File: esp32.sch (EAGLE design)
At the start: 28 parts, among them IC1 LM1117IMPX-3.3, U1 ESP32MOD

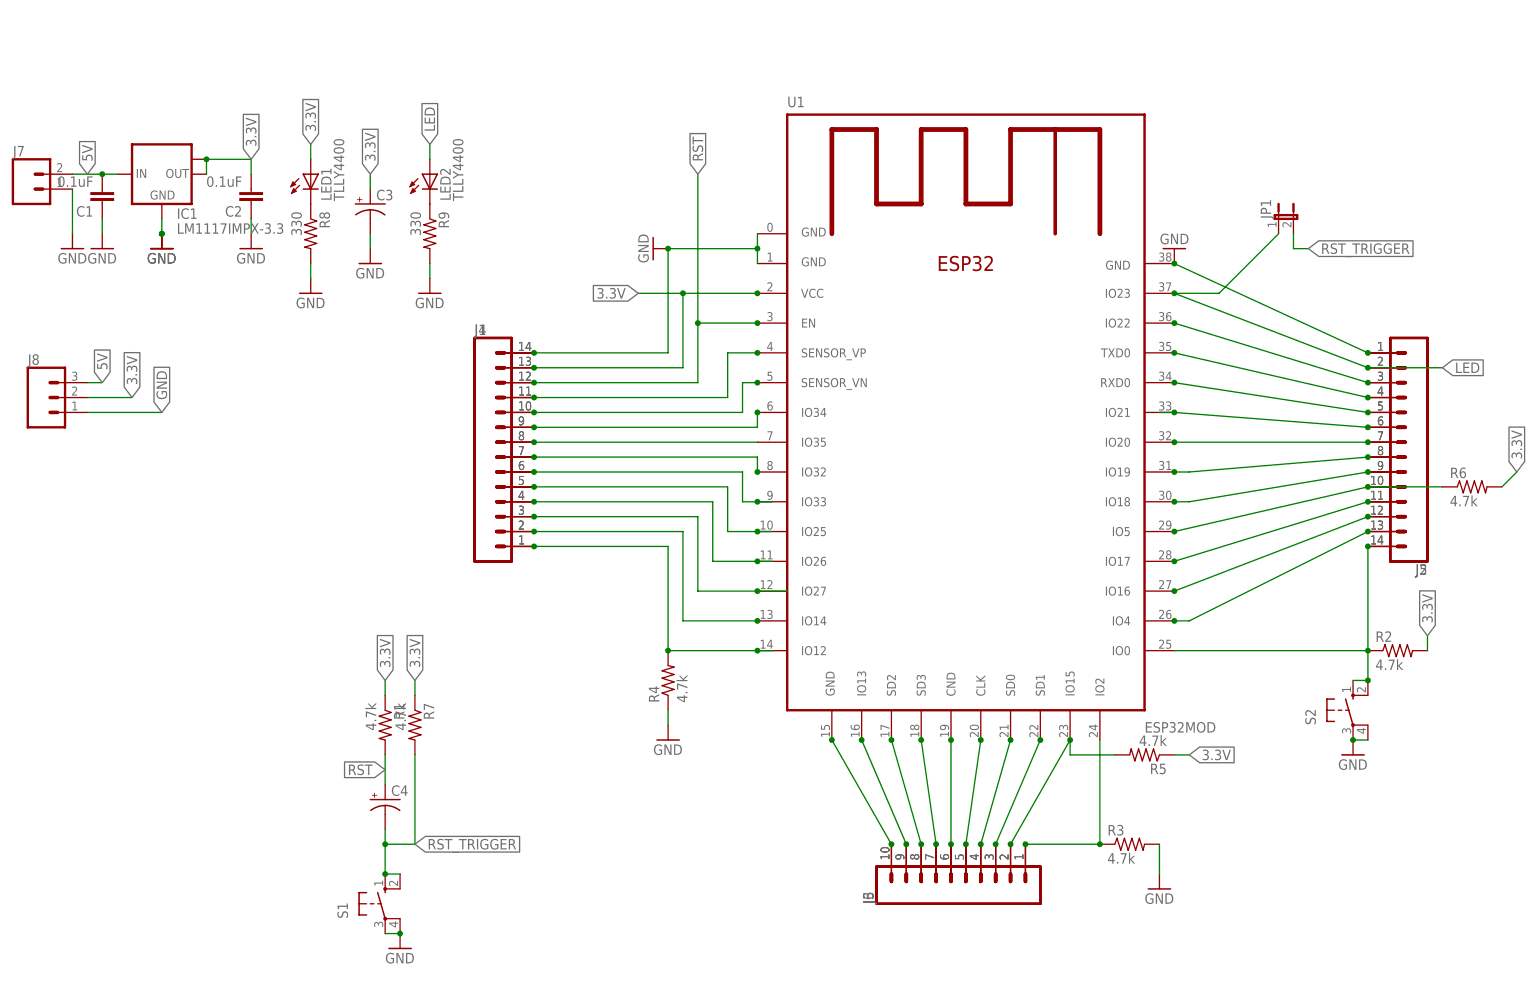
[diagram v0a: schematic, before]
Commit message: Finalized the layout with cheap design
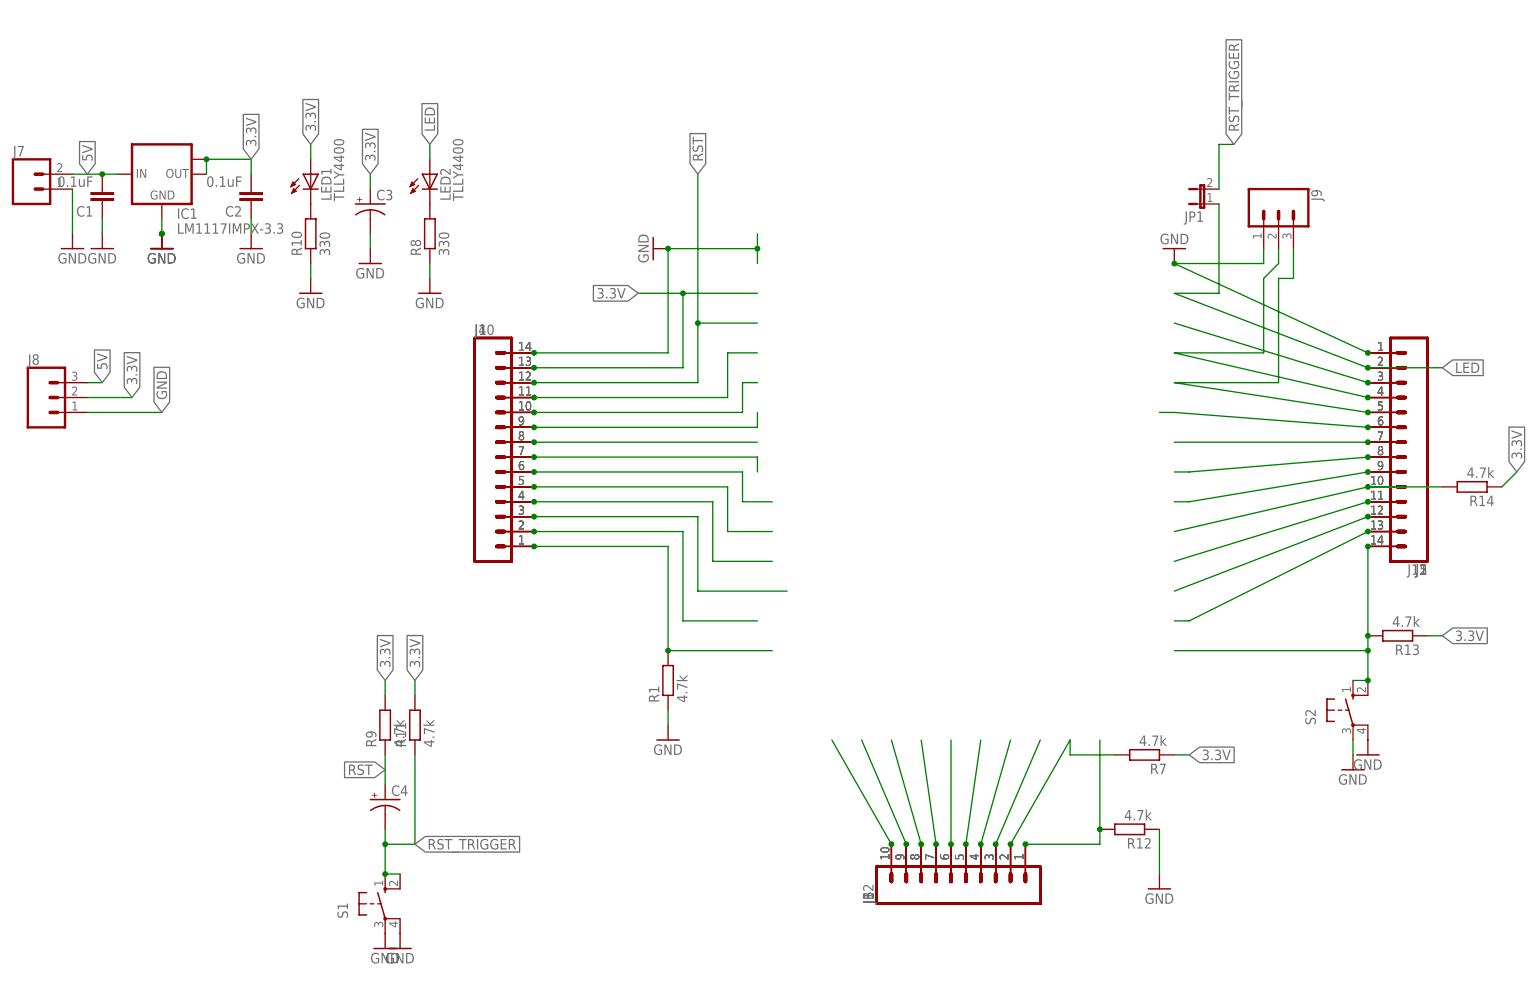
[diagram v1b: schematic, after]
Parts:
- removed R2, R3, R4, R5, R6: 4.7k, rcl:R-US_0411/15
- removed U1: ESP32MOD, ESP3x:ESP32MOD
- added J10, J11: (no value), SparkFun-Connectors:CONN_14LONGPADS
- added J12: (no value), SparkFun-Connectors:CONN_10"
- added J9: (no value), SparkFun-Connectors:CONN_03
- added R10: 330, rcl:R-EU_0207/12
- added R11, R12, R13, R14: 4.7k, rcl:R-EU_0207/12
- R1, R7, R8: device rcl:R-US_0411/15 -> rcl:R-EU_0207/12
- R9: value 330 -> 4.7k; device rcl:R-US_0411/15 -> rcl:R-EU_0207/12
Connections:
- net 3.3V: now also J10.13, R11.2, R13.1, R14.1, R9.2; no longer R1.1, R2.2, R5.1, R6.2, U1.VCC
- net GND: now also J10.14, J11.1, J12.10, J9.1, R1.1, R10.1, R12.1, R8.1; no longer R3.2, R4.1, R8.2, R9.2, U1.GND, U1.GND@0, U1.GND@1, U1.GND@3
- net LED: now also J11.2; no longer U1.IO23
- net N$1: now also J11.7; no longer U1.IO20
- net N$10: now also J10.5; no longer U1.IO25
- net N$11: now also J10.4; no longer U1.IO26
- net N$12: now also J10.3; no longer U1.IO27
- net N$13: now also J10.2; no longer U1.IO14
- net N$14: now also J10.1, R1.2; no longer R4.2, U1.IO12
- net N$15: now also J11.5, J9.3; no longer U1.RXD0
- net N$16: now also J11.4, J9.2; no longer U1.TXD0
- net N$17: now also J11.3; no longer U1.IO22
- net N$19: now also J11.10, R14.2; no longer R6.1, U1.IO5
- net N$2: now also J10.11; no longer U1.SENSOR_VP
- net N$20: now also J11.6; no longer U1.IO21
- net N$22: now also J11.8; no longer U1.IO19
- net N$23: now also J11.9; no longer U1.IO18
- net N$25: now also J11.11; no longer U1.IO17
- net N$26: now also J11.12; no longer U1.IO16
- net N$27: now also J11.13; no longer U1.IO4
- net N$28: now also J11.14, R13.2; no longer R2.1, U1.IO0
- net N$3: now also J10.10; no longer U1.SENSOR_VN
- net N$30: now also J12.9; no longer U1.IO13
- net N$31: now also J12.8; no longer U1.SD2
- net N$32: now also J12.7; no longer U1.SD3
- net N$33: now also J12.6; no longer U1.CND
- net N$34: now also J12.5; no longer U1.CLK
- net N$35: now also J12.4; no longer U1.SD0
- net N$36: now also J12.3; no longer U1.SD1
- net N$37: now also J12.2, R7.2; no longer R5.2, U1.IO15
- net N$38: now also J12.1, R12.2; no longer R3.1, U1.IO2
- net N$4: now also R10.2; no longer R8.1
- net N$5: now also R8.2; no longer R9.1
- net N$6: now also J10.9; no longer U1.IO34
- net N$7: now also J10.8; no longer U1.IO35
- net N$8: now also J10.7; no longer U1.IO32
- net N$9: now also J10.6; no longer U1.IO33
- net RST: now also J10.12, R9.1; no longer R1.2, U1.EN
- net RST_TRIGGER: now also R11.1; no longer R7.2
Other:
- moved on the sheet: JP1
